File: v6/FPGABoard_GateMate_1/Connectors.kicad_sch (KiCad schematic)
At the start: 21 parts, among them IC1 TXB0108RUKR, IC2 TXB0108RUKR, IC3 TXB0108RUKR, IC4 TXB0108RUKR, J3 Conn_02x16_Odd_Even, J4 Conn_02x16_Odd_Even, J5 Conn_02x16_Odd_Even, J6 Conn_02x04_Odd_Even, J7 Conn_02x04_Odd_Even

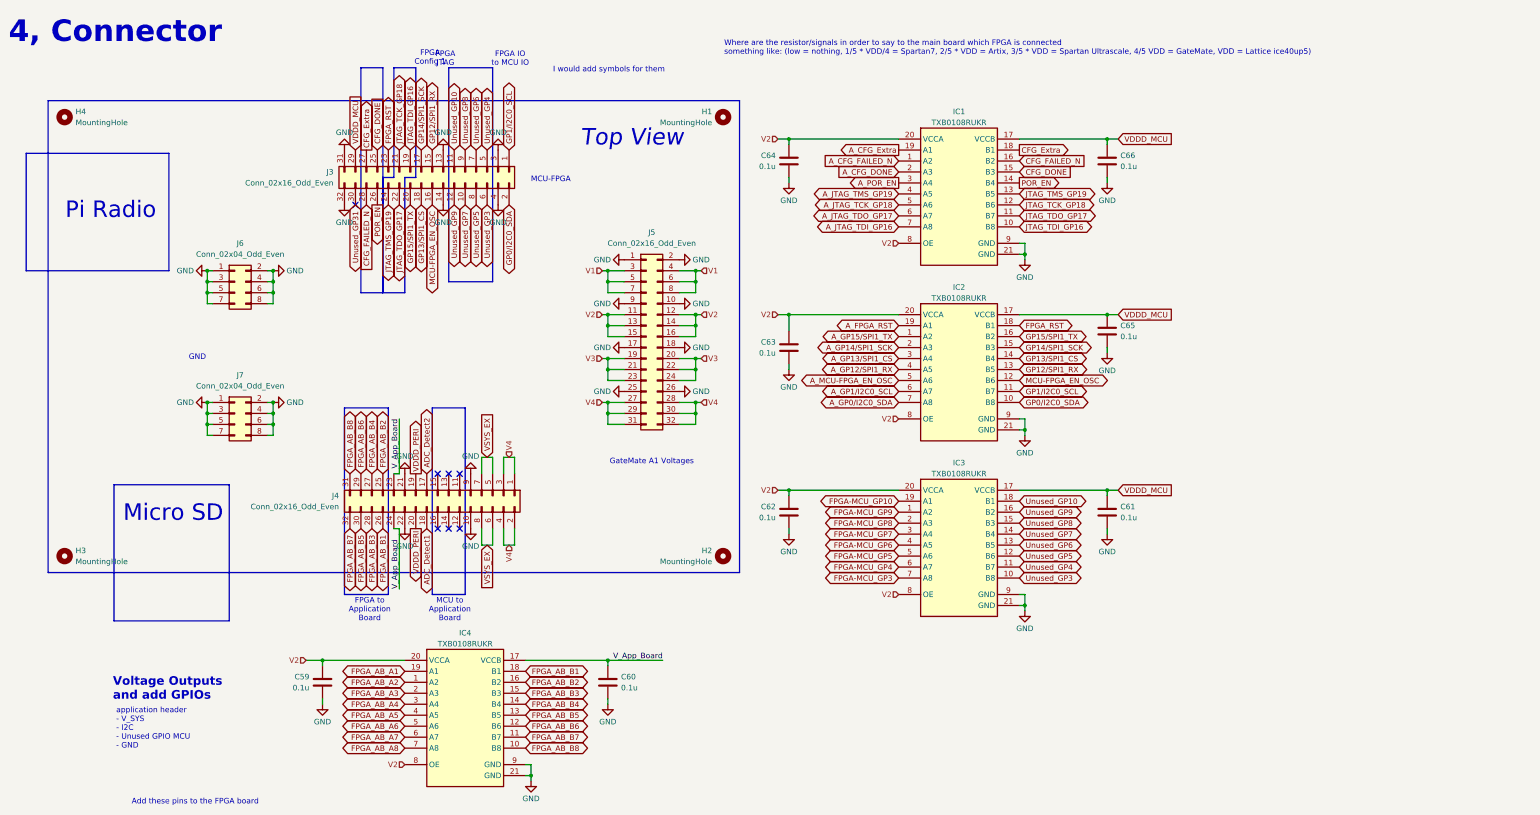
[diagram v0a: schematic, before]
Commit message: Fix small errors for the design
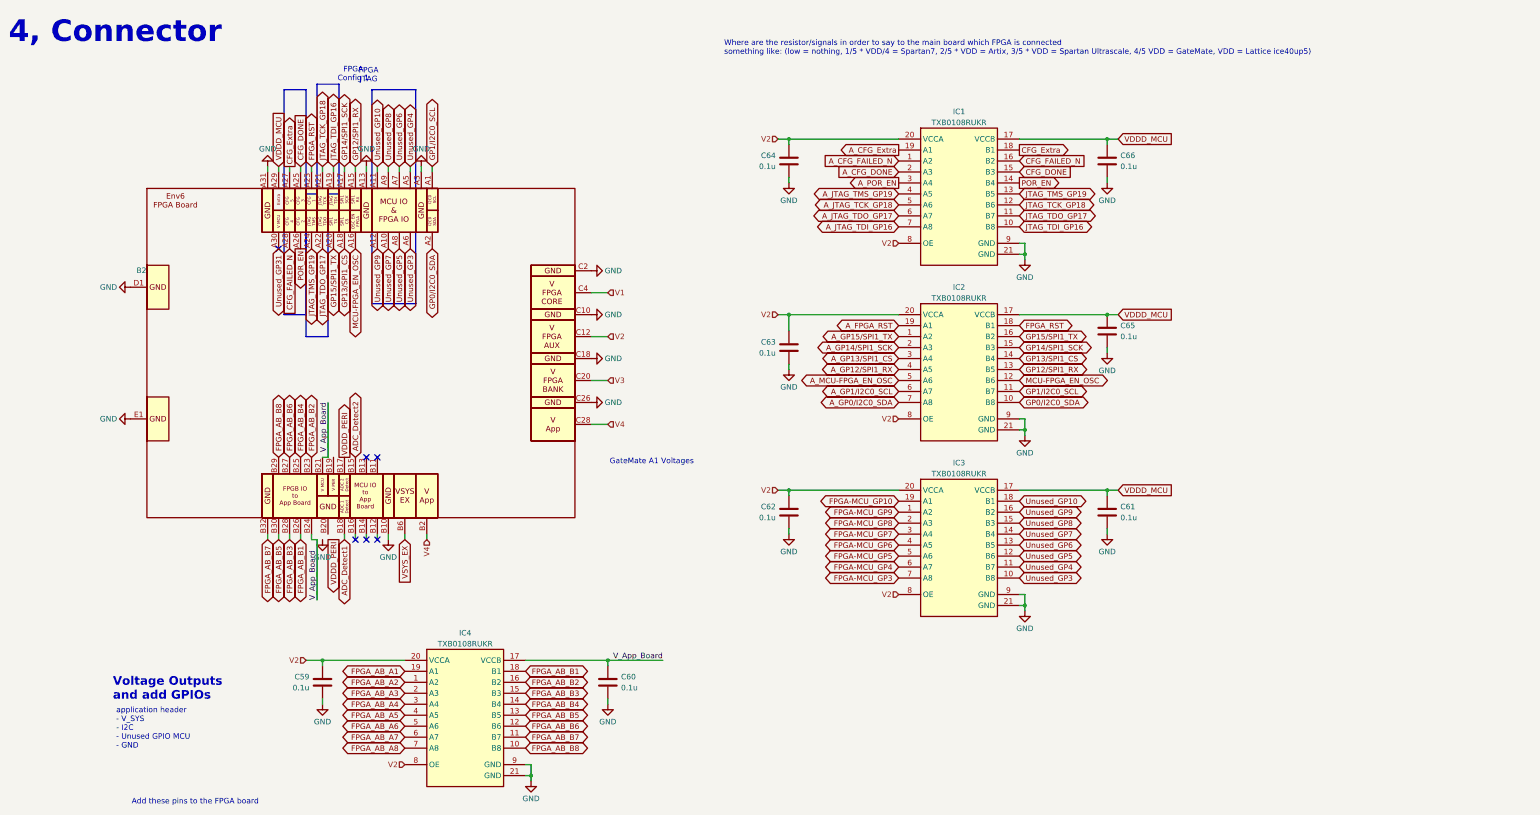
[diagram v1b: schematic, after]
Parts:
- removed H1, H2, H3, H4: MountingHole, MountingHole:MountingHole_2.5mm, symbol Mechanical:MountingHole
- removed J3, J4, J5: Conn_02x16_Odd_Even, Connector_PinHeader_2.00mm:PinHeader_2x16_P2.00mm_Vertical, symbol Connector_Generic:Conn_02x16_Odd_Even
- removed J6, J7: Conn_02x04_Odd_Even, Connector_PinHeader_2.00mm:PinHeader_2x04_P2.00mm_Vertical, symbol Connector_Generic:Conn_02x04_Odd_Even
- added B2: (no value), ENv6_Custom_Footprints:ExtensionBoard_ENv6, symbol ENv6_Custom_Symbols:FPGABoard_ENv6
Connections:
- net ADC_Detect1: now also B2.B18
- net ADC_Detect2: now also B2.B15
- net CFG_DONE: now also B2.A25
- net CFG_Extra: now also B2.A27
- net CFG_FAILED_N: now also B2.A28
- net FPGA_AB_B1: now also B2.B26
- net FPGA_AB_B2: now also B2.B23
- net FPGA_AB_B3: now also B2.B28
- net FPGA_AB_B4: now also B2.B25
- net FPGA_AB_B5: now also B2.B30
- net FPGA_AB_B6: now also B2.B27
- net FPGA_AB_B7: now also B2.B31, B2.B32
- net FPGA_AB_B8: now also B2.B29
- net FPGA_RST: now also B2.A23
- net GND: now also B2.A13, B2.A14, B2.A3, B2.A31, B2.A32, B2.A4, B2.B10, B2.B9, B2.C1, B2.C10, B2.C17, B2.C18, B2.C2, B2.C25, B2.C26, B2.C9, B2.D1, B2.D2, B2.D3, B2.D4, B2.D5, B2.D6, B2.D7, B2.D8, B2.E1, B2.E2, B2.E3, B2.E4, B2.E5, B2.E6, B2.E7, B2.E8
- net GP0/I2C0_SDA: now also B2.A2
- net GP12/SPI1_RX: now also B2.A15
- net GP13/SPI1_CS: now also B2.A18
- net GP14/SPI1_SCK: now also B2.A17
- net GP15/SPI1_TX: now also B2.A20
- net GP1/I2C0_SCL: now also B2.A1
- net JTAG_TCK_GP18: now also B2.A21
- net JTAG_TDI_GP16: now also B2.A19
- net JTAG_TDO_GP17: now also B2.A22
- net JTAG_TMS_GP19: now also B2.A24
- net MCU-FPGA_EN_OSC: now also B2.A16
- net POR_EN: now also B2.A26
- net Unused_GP10: now also B2.A11
- net Unused_GP3: now also B2.A6
- net Unused_GP31: now also B2.A30
- net Unused_GP4: now also B2.A5
- net Unused_GP5: now also B2.A8
- net Unused_GP6: now also B2.A7
- net Unused_GP7: now also B2.A10
- net Unused_GP8: now also B2.A9
- net Unused_GP9: now also B2.A12
- net V1: now also B2.C3, B2.C4, B2.C5, B2.C6, B2.C7, B2.C8
- net V2: now also B2.C11, B2.C12, B2.C13, B2.C14, B2.C15, B2.C16
- net V3: now also B2.C19, B2.C20, B2.C21, B2.C22, B2.C23, B2.C24
- net V4: now also B2.B1, B2.B2, B2.B3, B2.B4, B2.C27, B2.C28, B2.C29, B2.C30, B2.C31, B2.C32
- net VDDD_MCU: now also B2.A29
- net VDDD_PERI: now also B2.B17
- net VSYS_EX: now also B2.B5, B2.B6, B2.B7, B2.B8
- net V_App_Board: now also B2.B21, B2.B24
- new net: B2.B20, B2.B22
- no-connect marks 7 -> 6
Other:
- note removed: "FPGA IO to MCU IO"
- note removed: "FPGA to Application Board"
- note removed: "GND"
- note removed: "I would add symbols for them"
- note removed: "MCU to Application Board"
- note removed: "MCU-FPGA"
- note removed: "Micro SD"
- note removed: "Pi Radio"
- note removed: "Top View"
